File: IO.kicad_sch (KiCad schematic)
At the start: 15 parts, among them J502 I2C, J503 SPI, J601 JST_SHBM04B-SRSS-TB, SW501 TS-1010A-B, SW601 B3U-3100-P, U602 SN74LVC1G14DBVR

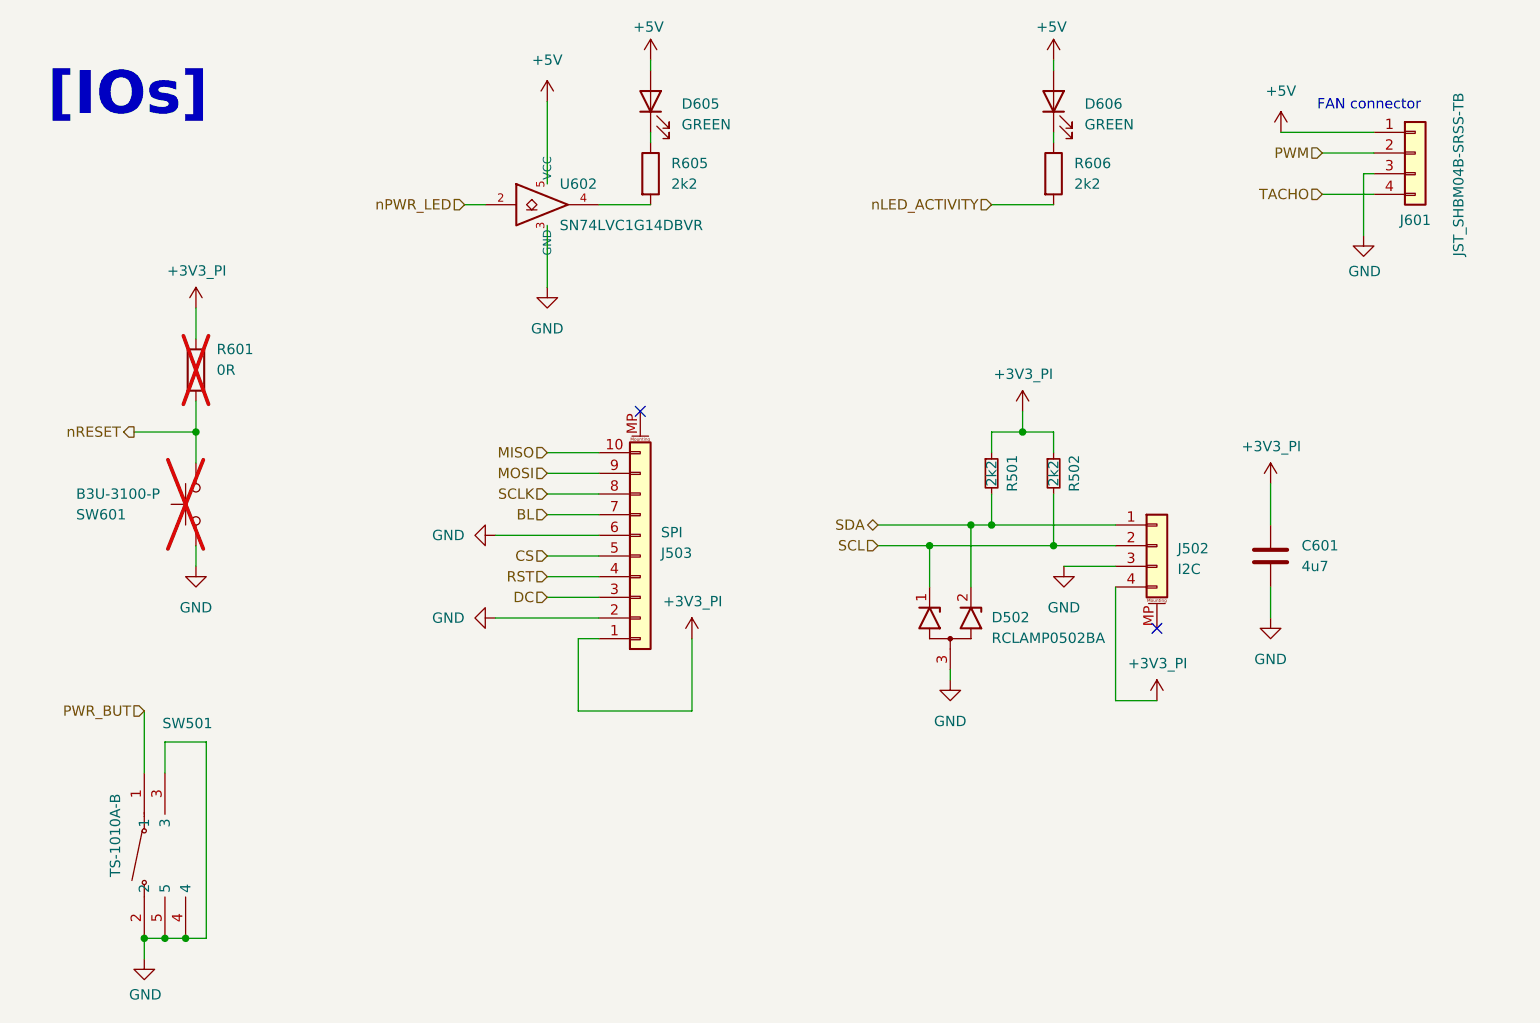
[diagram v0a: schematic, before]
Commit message: vias
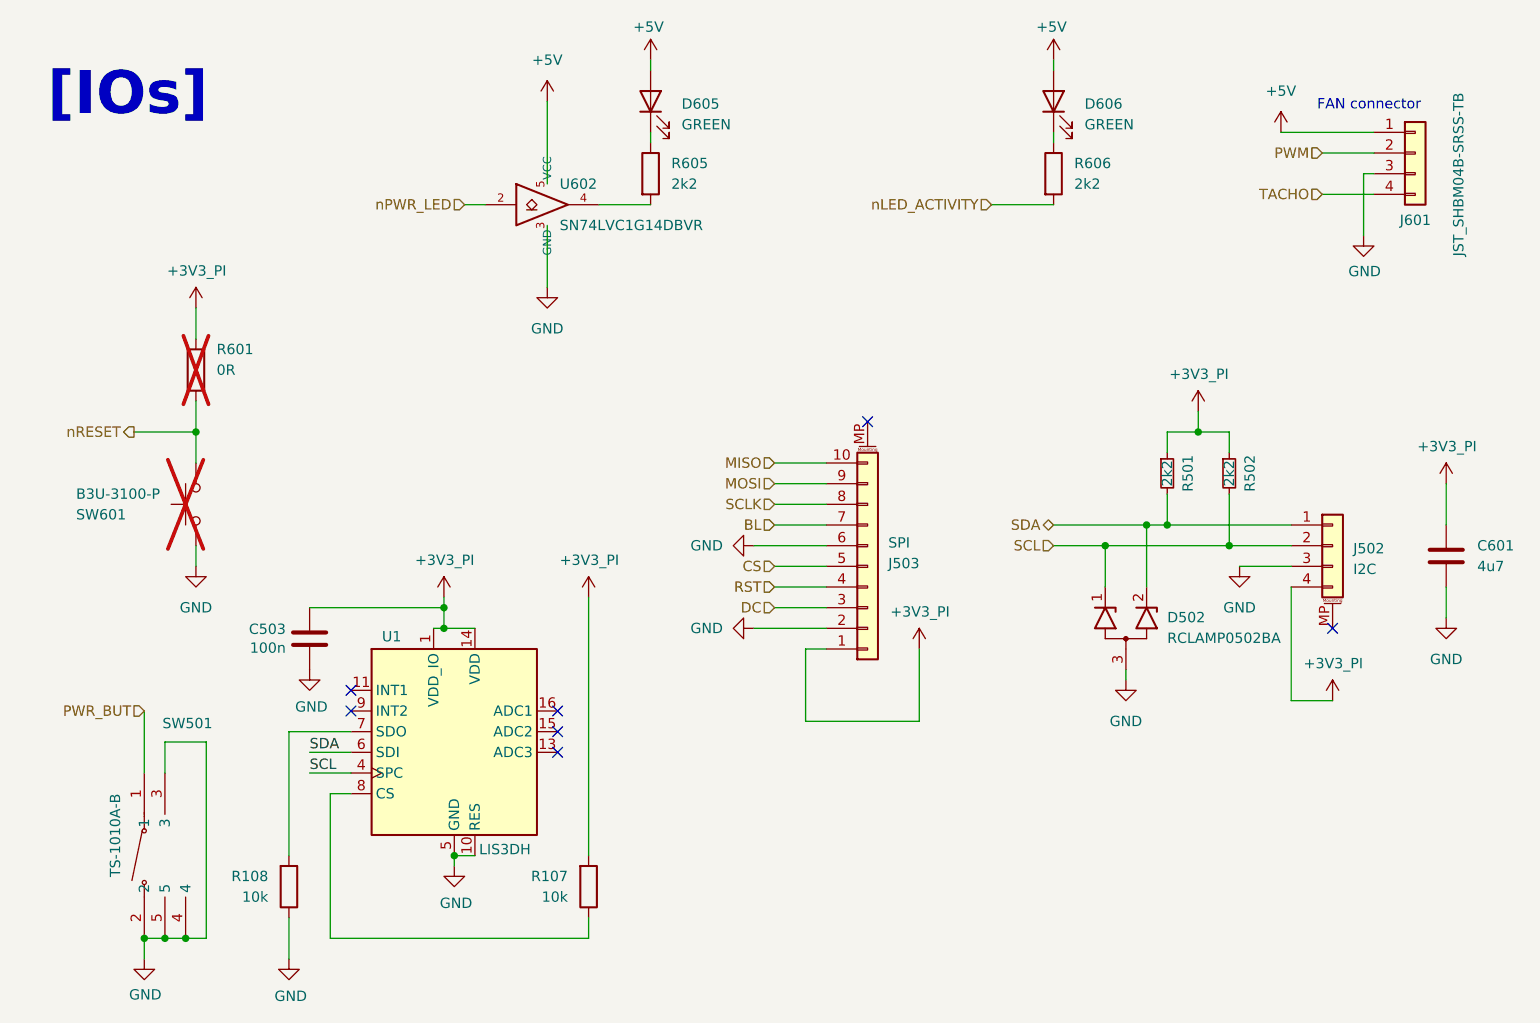
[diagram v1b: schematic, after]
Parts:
- added C503: 100n, Capacitor_SMD:C_0402_1005Metric, symbol Device:C
- added R107, R108: 10k, Resistor_SMD:R_0402_1005Metric, symbol Device:R
- added U1: LIS3DH, Package_LGA:LGA-16_3x3mm_P0.5mm_LayoutBorder3x5y, symbol Sensor_Motion:LIS3DH
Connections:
- net +3V3_PI: now also C503.1, R107.2, U1.1 (VDD_IO), U1.14 (VDD)
- net GND: now also C503.2, R108.1, U1.10 (RES), U1.12 (GND), U1.5 (GND)
- net SCL: now also U1.4 (SPC)
- net SDA: now also U1.6 (SDI)
- new net: R108.2, U1.7 (SDO)
- new net: R107.1, U1.8 (CS)
- no-connect marks 2 -> 7
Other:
- moved on the sheet: C601, D502, J502, J503, R501, R502
